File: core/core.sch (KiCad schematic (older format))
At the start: 211 parts, among them K0 KEYSW, K1 KEYSW, K10 KEYSW, K11 KEYSW, K12 KEYSW, K13 KEYSW, K14 KEYSW, K15 KEYSW, K16 KEYSW, K17 KEYSW, K18 KEYSW, K19 KEYSW, K2 KEYSW, K20 KEYSW, K21 KEYSW, K22 KEYSW, K23 KEYSW, K24 KEYSW, K25 KEYSW, K26 KEYSW, K27 KEYSW, K28 KEYSW, K29 KEYSW, K3 KEYSW, K30 KEYSW, K31 KEYSW, K32 KEYSW, K33 KEYSW, K34 KEYSW, K35 KEYSW, K36 KEYSW, K37 KEYSW, K38 KEYSW, K39 KEYSW, K4 KEYSW, K40 KEYSW, K41 KEYSW, K42 KEYSW, K43 KEYSW, K44 KEYSW, K45 KEYSW, K46 KEYSW, K47 KEYSW, K48 KEYSW, K49 KEYSW, K5 KEYSW, K50 KEYSW, K51 KEYSW, K52 KEYSW, K53 KEYSW, K54 KEYSW, K55 KEYSW, K56 KEYSW, K57 KEYSW, K58 KEYSW, K59 KEYSW, K6 KEYSW, K60 KEYSW, K61 KEYSW, K62 KEYSW, K63 KEYSW, K64 KEYSW, K65 KEYSW, K66 KEYSW, K67 KEYSW, K68 KEYSW, K69 KEYSW, K7 KEYSW, K8 KEYSW, K9 KEYSW, U1 TEENSY2.0

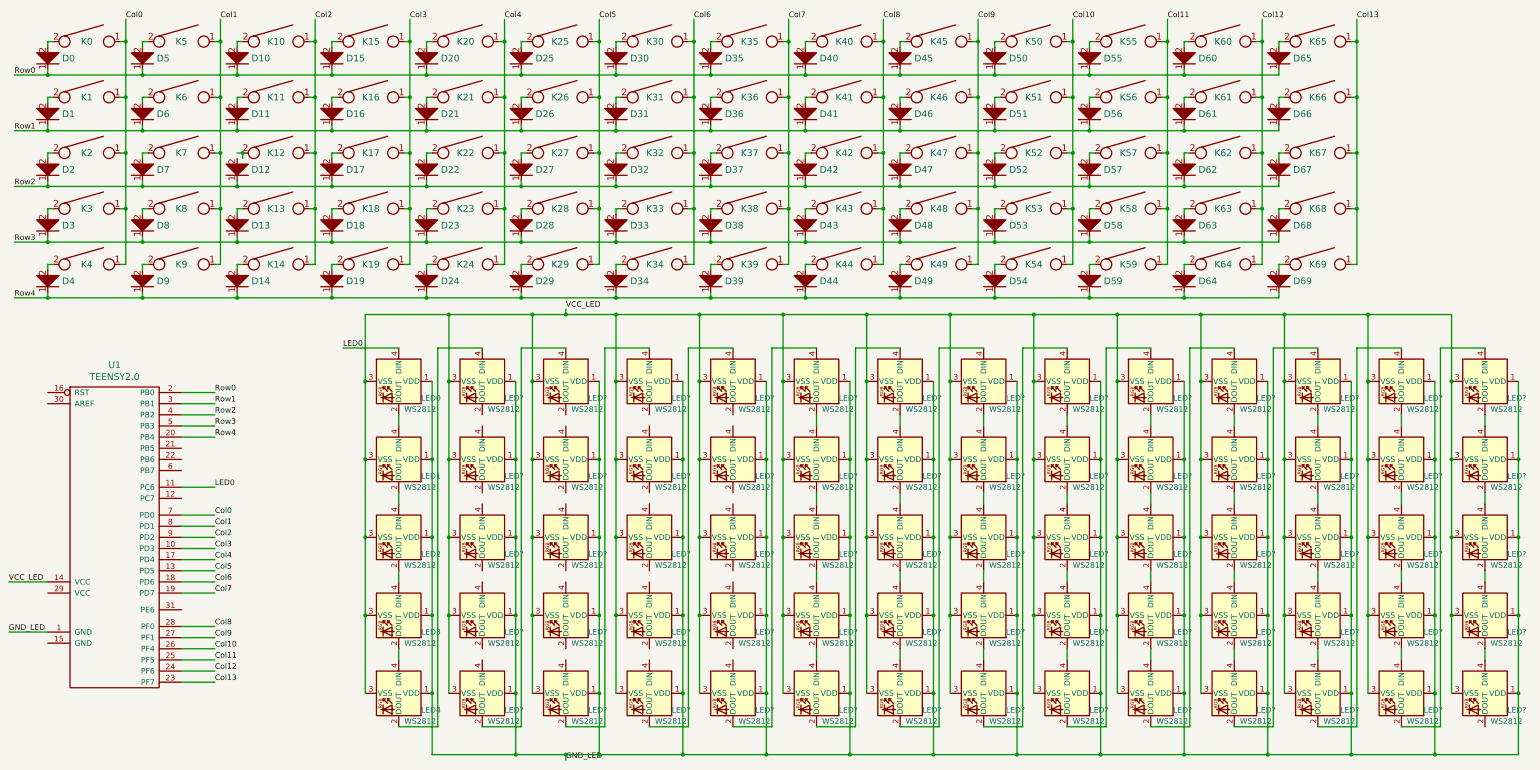
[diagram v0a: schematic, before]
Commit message: investigate 3mm rgb leds
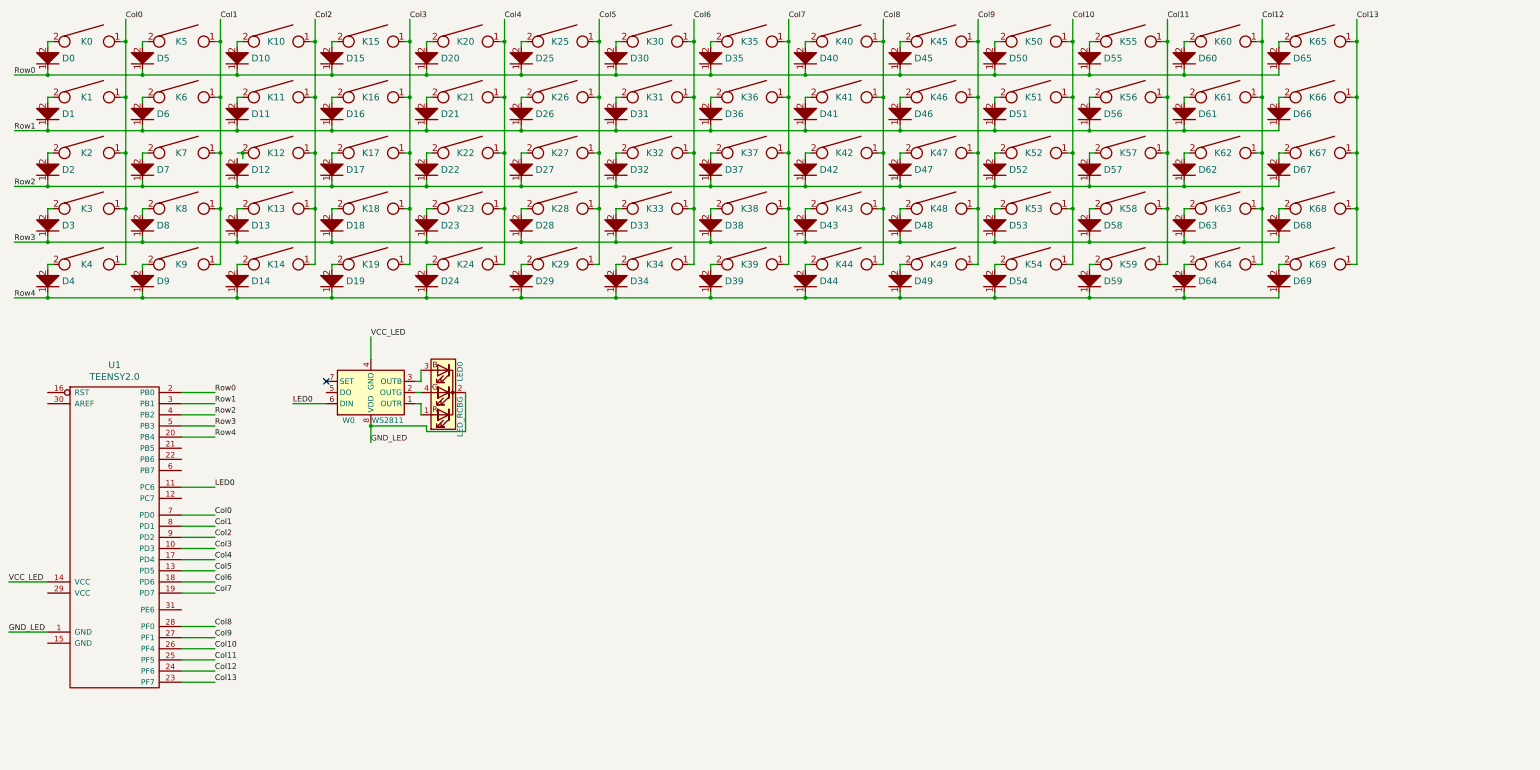
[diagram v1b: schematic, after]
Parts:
- removed LED0, LED1, LED2, LED3, LED4, LED? (x65): WS2812, LED_SMD:LED_WS2812B_PLCC4_5.0x5.0mm_P3.2mm, symbol LED:WS2812B
- added LED0: LED_RCBG, Connector_PinHeader_1.00mm:PinHeader_1x04_P1.00mm_Horizontal, symbol Device:LED_RCBG
- added W0: WS2811, Package_SO:SOIC-8-1EP_3.9x4.9mm_P1.27mm_EP2.29x3mm, symbol Driver_LED:WS2811
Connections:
- net GND_LED: now also LED0.2 (K), W0.8 (VDD)
- net LED0: now also W0.6 (DIN)
- net VCC_LED: now also W0.4 (GND)
- new net: LED0.1 (RA), W0.1 (OUTR)
- new net: LED0.4 (GA), W0.2 (OUTG)
- new net: LED0.3 (BA), W0.3 (OUTB)
- no-connect marks 0 -> 1
